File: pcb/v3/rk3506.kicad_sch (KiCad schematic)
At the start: 17 parts, among them J1 TestPoint, J15 TestPoint, J2 Conn_01x03, J3 TestPoint, U1 SOM3562_18

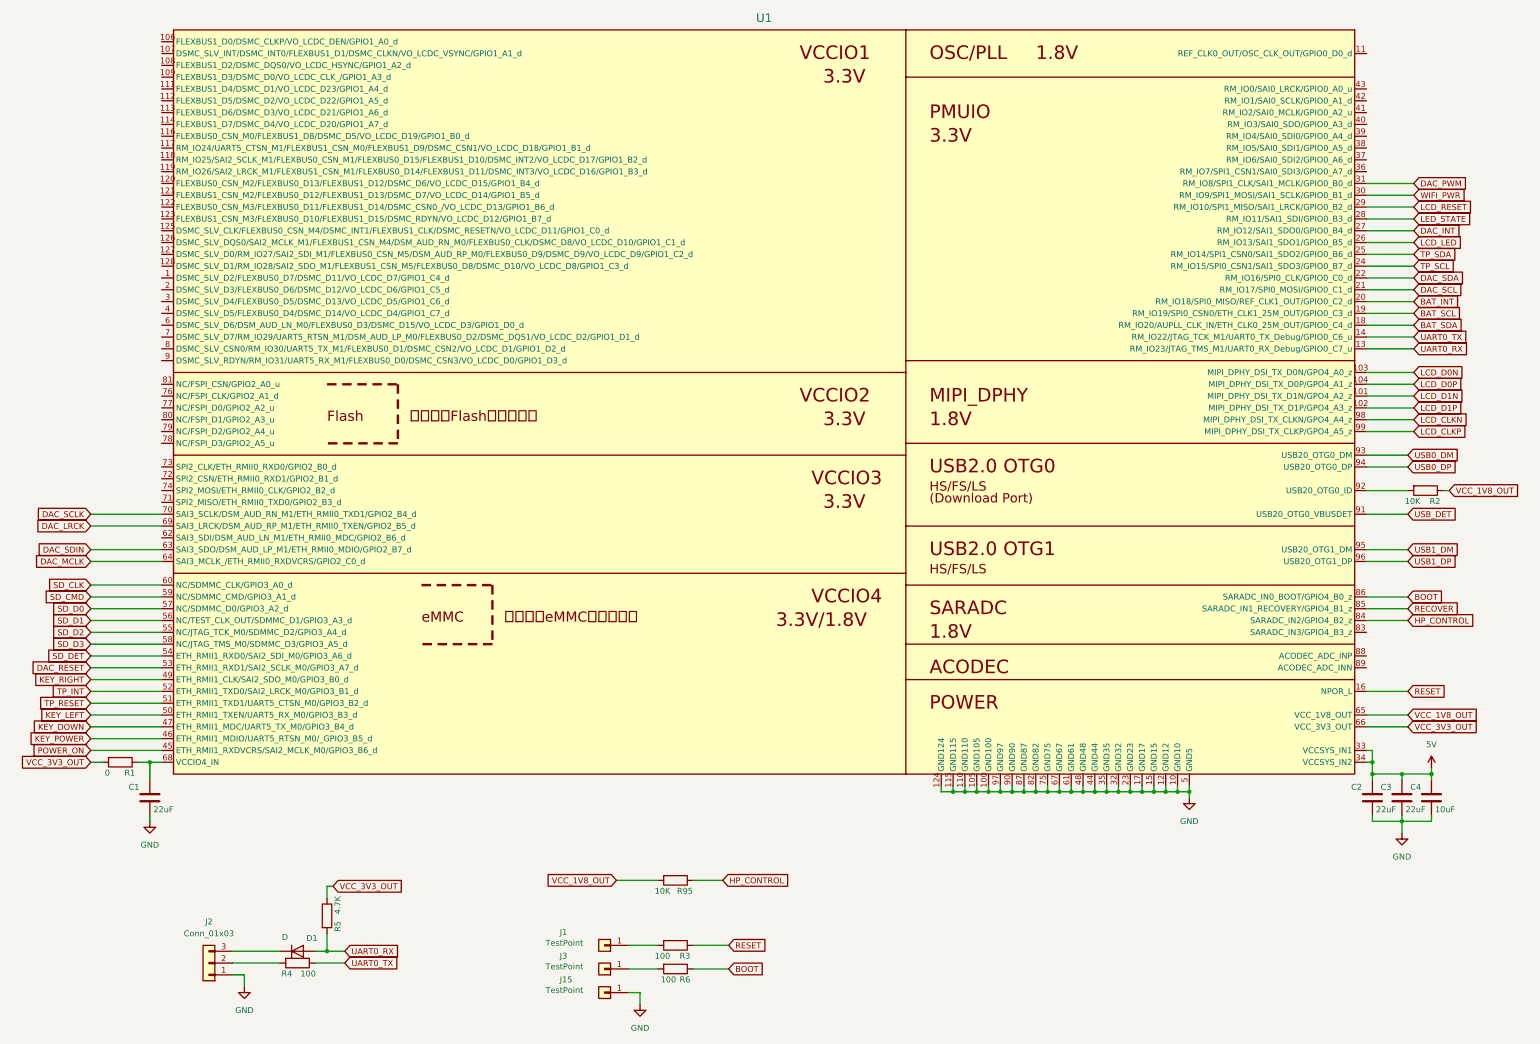
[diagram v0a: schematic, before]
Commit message: up
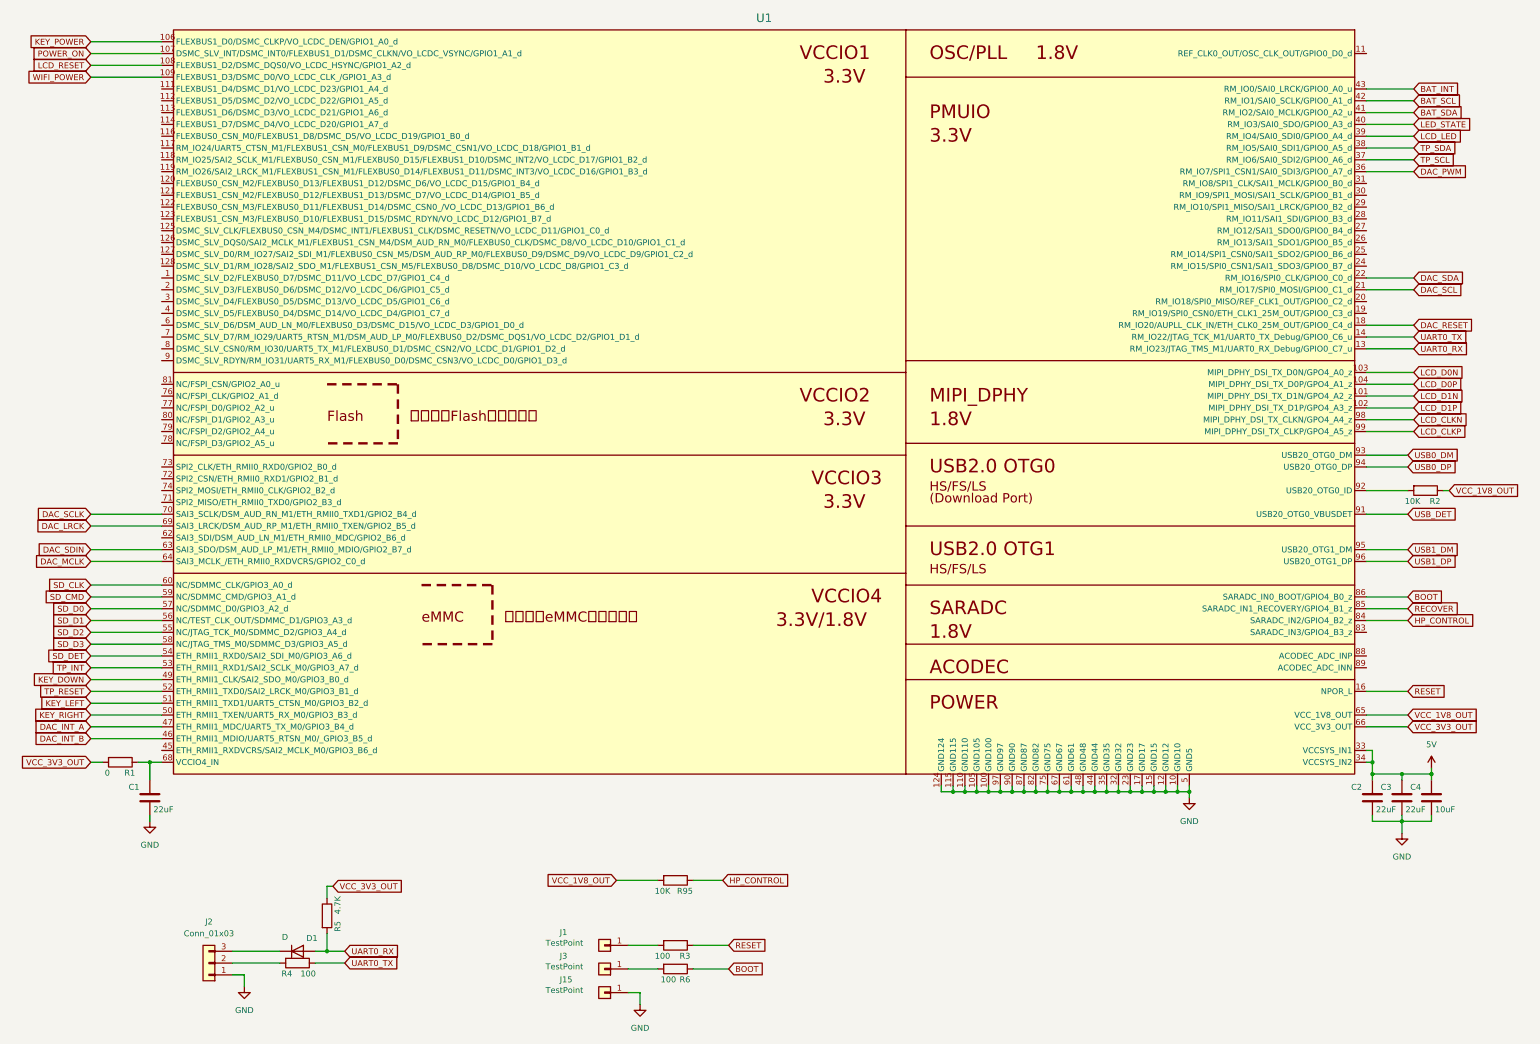
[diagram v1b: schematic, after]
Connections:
- net BAT_INT: now also U1.43 (RM_IO0/SAI0_LRCK/GPIO0_A0_u); no longer U1.20 (RM_IO18/SPI0_MISO/REF_CLK1_OUT/GPIO0_C2_d)
- net BAT_SCL: now also U1.42 (RM_IO1/SAI0_SCLK/GPIO0_A1_d); no longer U1.19 (RM_IO19/SPI0_CSN0/ETH_CLK1_25M_OUT/GPIO0_C3_d)
- net BAT_SDA: now also U1.41 (RM_IO2/SAI0_MCLK/GPIO0_A2_u); no longer U1.18 (RM_IO20/AUPLL_CLK_IN/ETH_CLK0_25M_OUT/GPIO0_C4_d)
- net DAC_PWM: now also U1.36 (RM_IO7/SPI1_CSN1/SAI0_SDI3/GPIO0_A7_d); no longer U1.31 (RM_IO8/SPI1_CLK/SAI1_MCLK/GPIO0_B0_d)
- net DAC_RESET: now also U1.18 (RM_IO20/AUPLL_CLK_IN/ETH_CLK0_25M_OUT/GPIO0_C4_d); no longer U1.53 (ETH_RMII1_RXD1/SAI2_SCLK_M0/GPIO3_A7_d)
- net KEY_DOWN: now also U1.49 (ETH_RMII1_CLK/SAI2_SDO_M0/GPIO3_B0_d); no longer U1.47 (ETH_RMII1_MDC/UART5_TX_M0/GPIO3_B4_d)
- net KEY_LEFT: now also U1.51 (ETH_RMII1_TXD1/UART5_CTSN_M0/GPIO3_B2_d); no longer U1.50 (ETH_RMII1_TXEN/UART5_RX_M0/GPIO3_B3_d)
- net KEY_POWER: now also U1.106 (FLEXBUS1_D0/DSMC_CLKP/VO_LCDC_DEN/GPIO1_A0_d); no longer U1.46 (ETH_RMII1_MDIO/UART5_RTSN_M0/_GPIO3_B5_d)
- net KEY_RIGHT: now also U1.50 (ETH_RMII1_TXEN/UART5_RX_M0/GPIO3_B3_d); no longer U1.49 (ETH_RMII1_CLK/SAI2_SDO_M0/GPIO3_B0_d)
- net LCD_LED: now also U1.39 (RM_IO4/SAI0_SDI0/GPIO0_A4_d); no longer U1.26 (RM_IO13/SAI1_SDO1/GPIO0_B5_d)
- net LCD_RESET: now also U1.108 (FLEXBUS1_D2/DSMC_DQS0/VO_LCDC_HSYNC/GPIO1_A2_d); no longer U1.29 (RM_IO10/SPI1_MISO/SAI1_LRCK/GPIO0_B2_d)
- net LED_STATE: now also U1.40 (RM_IO3/SAI0_SDO/GPIO0_A3_d); no longer U1.28 (RM_IO11/SAI1_SDI/GPIO0_B3_d)
- net POWER_ON: now also U1.107 (DSMC_SLV_INT/DSMC_INT0/FLEXBUS1_D1/DSMC_CLKN/VO_LCDC_VSYNC/GPIO1_A1_d); no longer U1.45 (ETH_RMII1_RXDVCRS/SAI2_MCLK_M0/GPIO3_B6_d)
- net TP_INT: now also U1.53 (ETH_RMII1_RXD1/SAI2_SCLK_M0/GPIO3_A7_d); no longer U1.52 (ETH_RMII1_TXD0/SAI2_LRCK_M0/GPIO3_B1_d)
- net TP_RESET: now also U1.52 (ETH_RMII1_TXD0/SAI2_LRCK_M0/GPIO3_B1_d); no longer U1.51 (ETH_RMII1_TXD1/UART5_CTSN_M0/GPIO3_B2_d)
- net TP_SCL: now also U1.37 (RM_IO6/SAI0_SDI2/GPIO0_A6_d); no longer U1.24 (RM_IO15/SPI0_CSN1/SAI1_SDO3/GPIO0_B7_d)
- net TP_SDA: now also U1.38 (RM_IO5/SAI0_SDI1/GPIO0_A5_d); no longer U1.25 (RM_IO14/SPI1_CSN0/SAI1_SDO2/GPIO0_B6_d)
- net WIFI_POWER: now reaches U1.109 (FLEXBUS1_D3/DSMC_D0/VO_LCDC_CLK_/GPIO1_A3_d)
- net DAC_INT: no longer names the net of U1.27 (RM_IO12/SAI1_SDO0/GPIO0_B4_d)
- net WIFI_PWR: no longer names the net of U1.30 (RM_IO9/SPI1_MOSI/SAI1_SCLK/GPIO0_B1_d)
- new net DAC_INT_A: U1.47 (ETH_RMII1_MDC/UART5_TX_M0/GPIO3_B4_d)
- new net DAC_INT_B: U1.46 (ETH_RMII1_MDIO/UART5_RTSN_M0/_GPIO3_B5_d)

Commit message: up
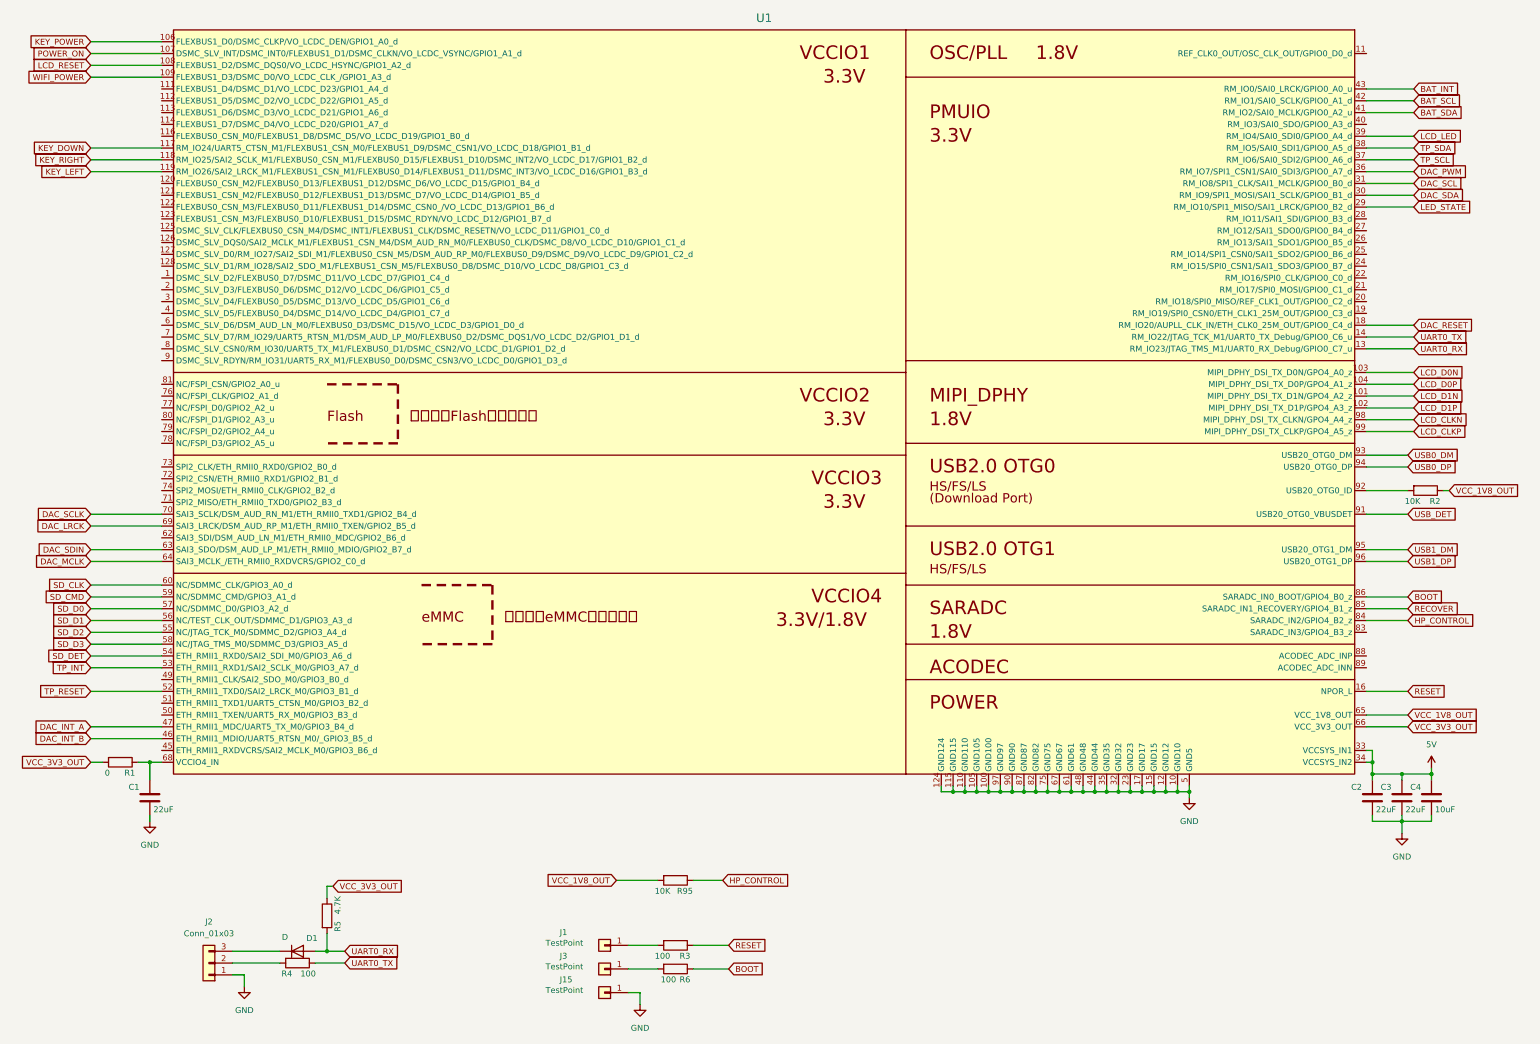
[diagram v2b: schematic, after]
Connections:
- net DAC_SCL: now also U1.31 (RM_IO8/SPI1_CLK/SAI1_MCLK/GPIO0_B0_d); no longer U1.21 (RM_IO17/SPI0_MOSI/GPIO0_C1_d)
- net DAC_SDA: now also U1.30 (RM_IO9/SPI1_MOSI/SAI1_SCLK/GPIO0_B1_d); no longer U1.22 (RM_IO16/SPI0_CLK/GPIO0_C0_d)
- net KEY_DOWN: now also U1.117 (RM_IO24/UART5_CTSN_M1/FLEXBUS1_CSN_M0/FLEXBUS1_D9/DSMC_CSN1/VO_LCDC_D18/GPIO1_B1_d); no longer U1.49 (ETH_RMII1_CLK/SAI2_SDO_M0/GPIO3_B0_d)
- net KEY_LEFT: now also U1.119 (RM_IO26/SAI2_LRCK_M1/FLEXBUS1_CSN_M1/FLEXBUS0_D14/FLEXBUS1_D11/DSMC_INT3/VO_LCDC_D16/GPIO1_B3_d); no longer U1.51 (ETH_RMII1_TXD1/UART5_CTSN_M0/GPIO3_B2_d)
- net KEY_RIGHT: now also U1.118 (RM_IO25/SAI2_SCLK_M1/FLEXBUS0_CSN_M1/FLEXBUS0_D15/FLEXBUS1_D10/DSMC_INT2/VO_LCDC_D17/GPIO1_B2_d); no longer U1.50 (ETH_RMII1_TXEN/UART5_RX_M0/GPIO3_B3_d)
- net LED_STATE: now also U1.29 (RM_IO10/SPI1_MISO/SAI1_LRCK/GPIO0_B2_d); no longer U1.40 (RM_IO3/SAI0_SDO/GPIO0_A3_d)

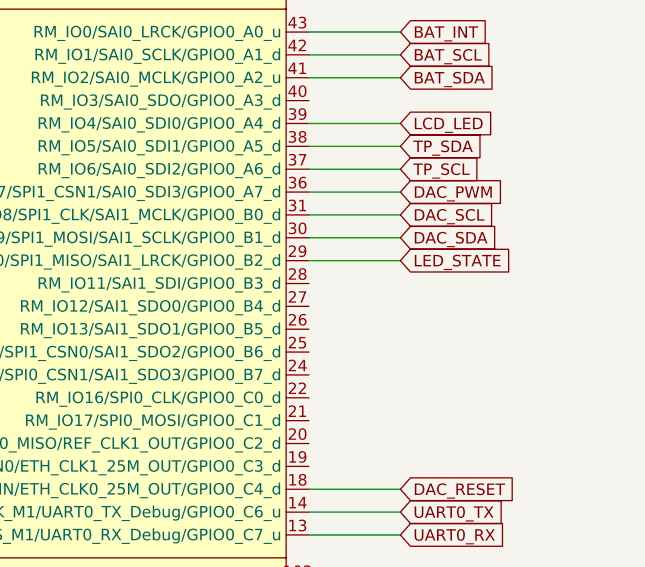
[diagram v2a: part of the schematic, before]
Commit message: up
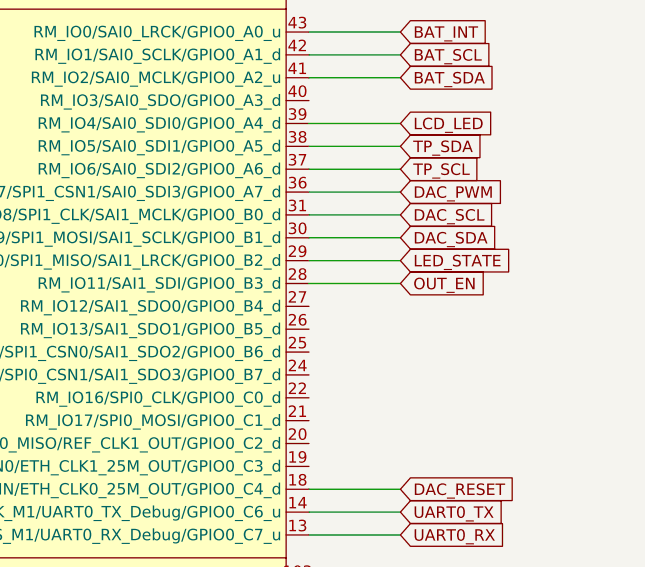
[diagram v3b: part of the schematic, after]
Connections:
- net OUT_EN: now reaches U1.28 (RM_IO11/SAI1_SDI/GPIO0_B3_d)
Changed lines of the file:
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@@
+	(wire
+		(pts
+			(xy 342.9 82.55) (xy 353.06 82.55)
+		)
+		(stroke
+			(width 0)
+			(type default)
+		)
+	)
 	(wire
 		(pts
@@
 			(effects
 				(font
+					(size 1.27 1.27)
+				)
+				(justify left)
+				(hide yes)
+			)
+		)
+	)
+	(global_label "OUT_EN"
+		(shape input)
+		(at 353.06 82.55 0)
+		(fields_autoplaced yes)
+		(effects
+			(font
+				(size 1.27 1.27)
+			)
+			(justify left)
+		)
+		(property "Intersheetrefs" "${INTERSHEET_REFS}"
+			(at 363.1209 82.55 0)
+			(effects
+				(font

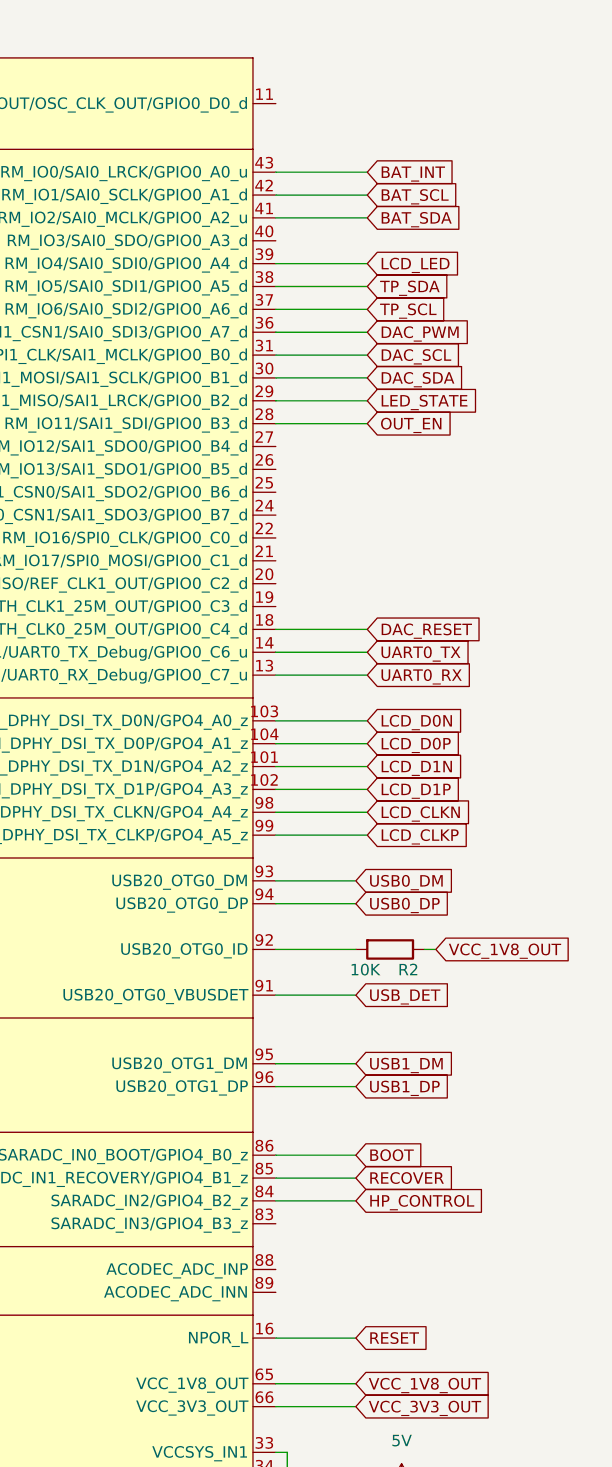
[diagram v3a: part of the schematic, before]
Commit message: up
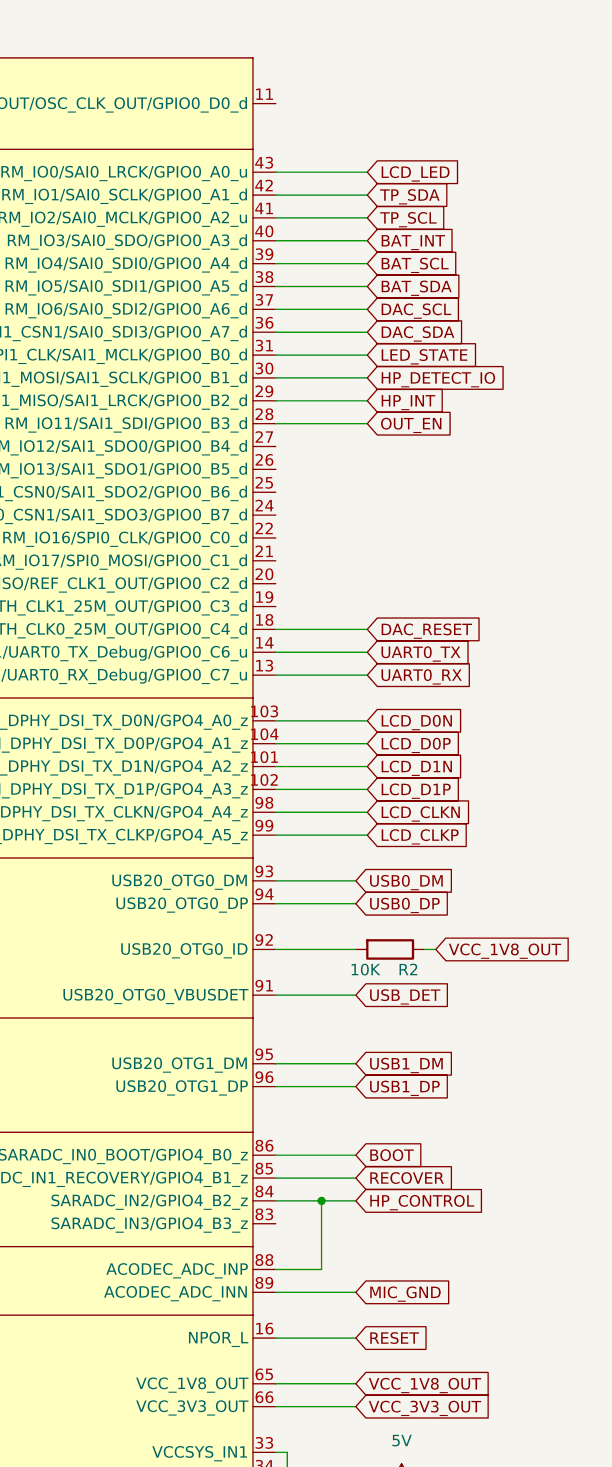
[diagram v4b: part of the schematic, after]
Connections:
- net DAC_PWM is gone; now on net DAC_SDA: U1.36 (RM_IO7/SPI1_CSN1/SAI0_SDI3/GPIO0_A7_d)
- net BAT_INT: now also U1.40 (RM_IO3/SAI0_SDO/GPIO0_A3_d); no longer U1.43 (RM_IO0/SAI0_LRCK/GPIO0_A0_u)
- net BAT_SCL: now also U1.39 (RM_IO4/SAI0_SDI0/GPIO0_A4_d); no longer U1.42 (RM_IO1/SAI0_SCLK/GPIO0_A1_d)
- net BAT_SDA: now also U1.38 (RM_IO5/SAI0_SDI1/GPIO0_A5_d); no longer U1.41 (RM_IO2/SAI0_MCLK/GPIO0_A2_u)
- net DAC_SCL: now also U1.37 (RM_IO6/SAI0_SDI2/GPIO0_A6_d); no longer U1.31 (RM_IO8/SPI1_CLK/SAI1_MCLK/GPIO0_B0_d)
- net DAC_SDA: no longer U1.30 (RM_IO9/SPI1_MOSI/SAI1_SCLK/GPIO0_B1_d)
- net HP_CONTROL: now also U1.88 (ACODEC_ADC_INP)
- net LCD_LED: now also U1.43 (RM_IO0/SAI0_LRCK/GPIO0_A0_u); no longer U1.39 (RM_IO4/SAI0_SDI0/GPIO0_A4_d)
- net LED_STATE: now also U1.31 (RM_IO8/SPI1_CLK/SAI1_MCLK/GPIO0_B0_d); no longer U1.29 (RM_IO10/SPI1_MISO/SAI1_LRCK/GPIO0_B2_d)
- net TP_SCL: now also U1.41 (RM_IO2/SAI0_MCLK/GPIO0_A2_u); no longer U1.37 (RM_IO6/SAI0_SDI2/GPIO0_A6_d)
- net TP_SDA: now also U1.42 (RM_IO1/SAI0_SCLK/GPIO0_A1_d); no longer U1.38 (RM_IO5/SAI0_SDI1/GPIO0_A5_d)
- net MIC_GND: now reaches U1.89 (ACODEC_ADC_INN)
- new net HP_DETECT_IO: U1.30 (RM_IO9/SPI1_MOSI/SAI1_SCLK/GPIO0_B1_d)
- new net HP_INT: U1.29 (RM_IO10/SPI1_MISO/SAI1_LRCK/GPIO0_B2_d)

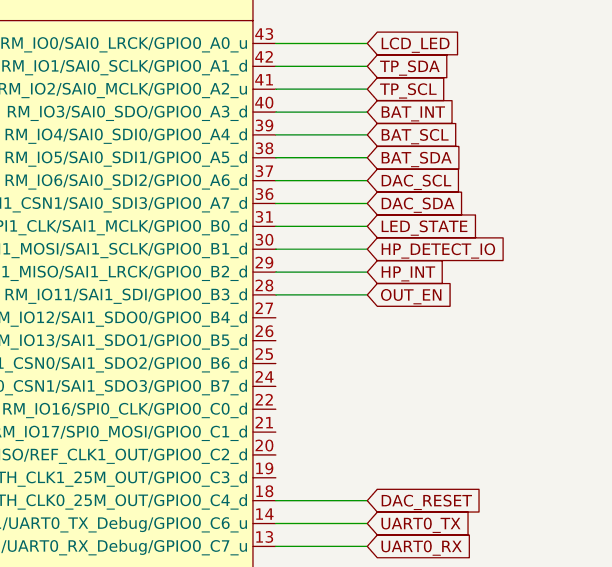
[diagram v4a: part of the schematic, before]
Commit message: up
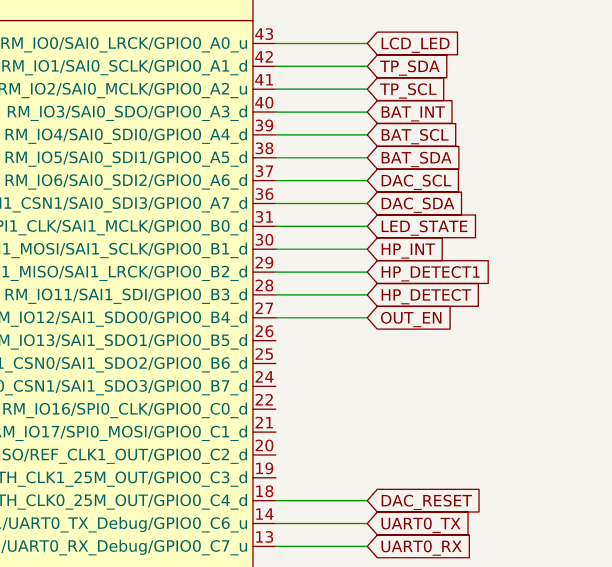
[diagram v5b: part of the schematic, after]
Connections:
- net HP_DETECT_IO is gone; now on net HP_INT: U1.30 (RM_IO9/SPI1_MOSI/SAI1_SCLK/GPIO0_B1_d)
- net HP_INT: no longer U1.29 (RM_IO10/SPI1_MISO/SAI1_LRCK/GPIO0_B2_d)
- net OUT_EN: now also U1.27 (RM_IO12/SAI1_SDO0/GPIO0_B4_d); no longer U1.28 (RM_IO11/SAI1_SDI/GPIO0_B3_d)
- new net HP_DETECT: U1.28 (RM_IO11/SAI1_SDI/GPIO0_B3_d)
- new net HP_DETECT1: U1.29 (RM_IO10/SPI1_MISO/SAI1_LRCK/GPIO0_B2_d)
